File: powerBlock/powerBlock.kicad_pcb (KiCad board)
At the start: 2 copper layers, 3 parts, among them U1 STM32F030C8Tx, U2 74HC164, U3 74HC164

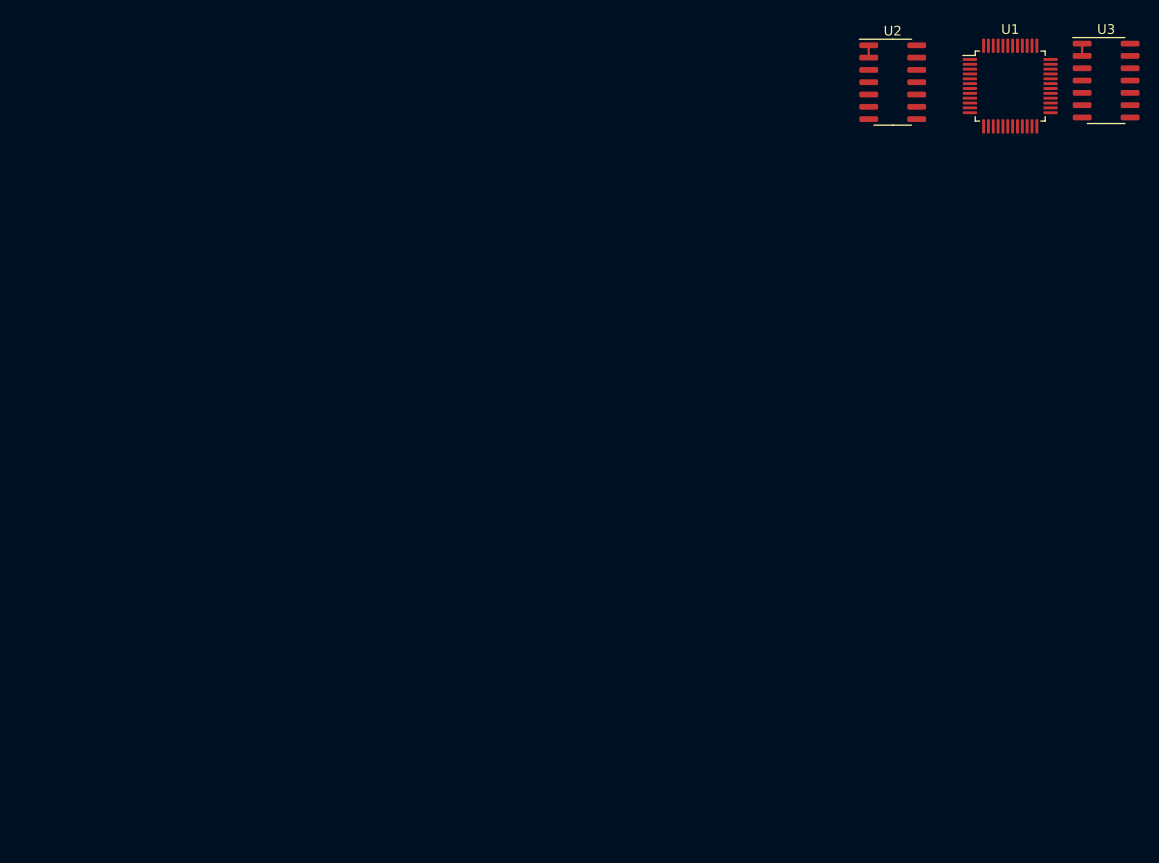
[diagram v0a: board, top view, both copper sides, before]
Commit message: Немного допилил схему. Немного оттрассировал
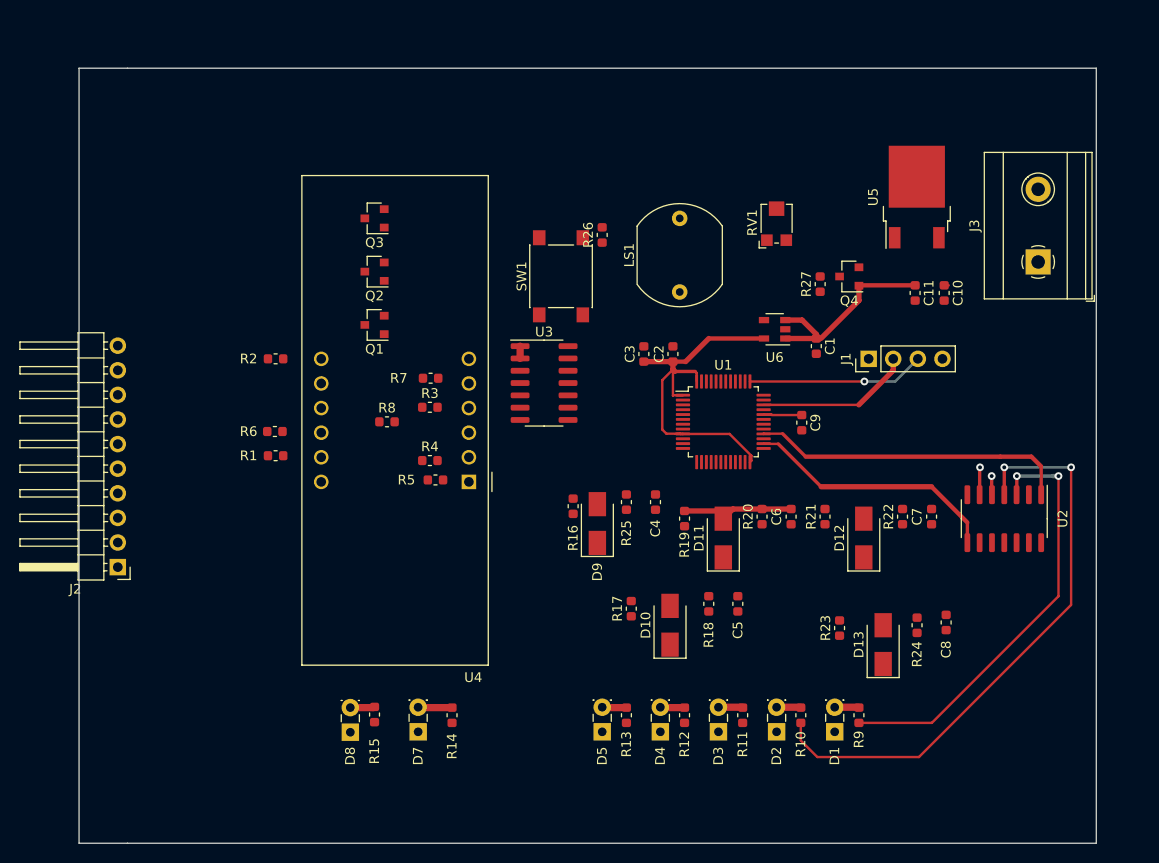
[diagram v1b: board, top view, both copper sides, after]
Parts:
- added C1: 10uF, Capacitor_SMD:C_0603_1608Metric, F.Cu at (111.1, 58.7)
- added C10: 10uF, Capacitor_SMD:C_0603_1608Metric, F.Cu at (124.3, 53.2)
- added C11: 10uF, Capacitor_SMD:C_0603_1608Metric, F.Cu at (121.3, 53.2)
- added C2: 100nF, Capacitor_SMD:C_0603_1608Metric, F.Cu at (96.3, 59.5)
- added C3: 100nF, Capacitor_SMD:C_0603_1608Metric, F.Cu at (93.3, 59.5)
- added C4: 1uF, Capacitor_SMD:C_0603_1608Metric, F.Cu at (94.5, 74.8)
- added C5: 1uF, Capacitor_SMD:C_0603_1608Metric, F.Cu at (103.0, 85.3)
- added C6: 1uF, Capacitor_SMD:C_0603_1608Metric, F.Cu at (108.5, 76.3)
- added C7: 1uF, Capacitor_SMD:C_0603_1608Metric, F.Cu at (123.0, 76.3)
- added C8: 1uF, Capacitor_SMD:C_0603_1608Metric, F.Cu at (124.5, 87.2)
- added C9: 1uF, Capacitor_SMD:C_0603_1608Metric, F.Cu at (109.6, 66.6)
- added D1: LED, LED_THT:LED_Rectangular_W3.9mm_H1.8mm, F.Cu at (113.0, 98.5)
- added D10: DO-214AC, Diode_SMD:D_SMA, F.Cu at (96.0, 87.5)
- added D11: DO-214AC, Diode_SMD:D_SMA, F.Cu at (101.5, 78.5)
- added D12: DO-214AC, Diode_SMD:D_SMA, F.Cu at (116.0, 78.5)
- added D13: DO-214AC, Diode_SMD:D_SMA, F.Cu at (118.0, 89.5)
- added D2: LED, LED_THT:LED_Rectangular_W3.9mm_H1.8mm, F.Cu at (107.0, 98.5)
- added D3: LED, LED_THT:LED_Rectangular_W3.9mm_H1.8mm, F.Cu at (101.0, 98.5)
- added D4: LED, LED_THT:LED_Rectangular_W3.9mm_H1.8mm, F.Cu at (95.0, 98.5)
- added D5: LED, LED_THT:LED_Rectangular_W3.9mm_H1.8mm, F.Cu at (89.0, 98.5)
- added D7: LED, LED_THT:LED_Rectangular_W3.9mm_H1.8mm, F.Cu at (70.0, 98.5)
- added D8: LED, LED_THT:LED_Rectangular_W3.9mm_H1.8mm, F.Cu at (63.0, 98.5)
- added D9: DO-214AC, Diode_SMD:D_SMA, F.Cu at (88.5, 77.0)
- added J1: Conn_01x04, Connector_PinHeader_2.54mm:PinHeader_1x04_P2.54mm_Vertical, F.Cu at (116.5, 60.0)
- added J2: Conn_01x10, Connector_PinHeader_2.54mm:PinHeader_1x10_P2.54mm_Horizontal, F.Cu at (39.0, 81.5)
- added J3: 282844-2, TerminalBlock_MetzConnect:TerminalBlock_MetzConnect_Type175_RT02702HBLC_1x02_P7.50mm_Horizontal, F.Cu at (134.0, 50.0)
- added LS1: Speaker_Crystal, OptoDevice:R_LDR_10x8.5mm_P7.6mm_Vertical, F.Cu at (97.0, 53.1)
- added Q1: BC857BMTF, Package_TO_SOT_SMD:SOT-23, F.Cu at (65.5, 56.5)
- added Q2: BC857BMTF, Package_TO_SOT_SMD:SOT-23, F.Cu at (65.5, 51.0)
- added Q3: BC857BMTF, Package_TO_SOT_SMD:SOT-23, F.Cu at (65.5, 45.5)
- added Q4: BC857BMTF, Package_TO_SOT_SMD:SOT-23, F.Cu at (114.5, 51.5)
- added R1: 18kOhm, Resistor_SMD:R_0603_1608Metric, F.Cu at (55.3, 70.0)
- added R10: 270, Resistor_SMD:R_0603_1608Metric, F.Cu at (109.5, 96.8)
- added R11: 270, Resistor_SMD:R_0603_1608Metric, F.Cu at (103.5, 96.8)
- added R12: 270, Resistor_SMD:R_0603_1608Metric, F.Cu at (97.5, 96.8)
- added R13: 270, Resistor_SMD:R_0603_1608Metric, F.Cu at (91.5, 96.8)
- added R14: 270, Resistor_SMD:R_0603_1608Metric, F.Cu at (73.5, 96.8)
- added R15: 270, Resistor_SMD:R_0603_1608Metric, F.Cu at (65.5, 96.7)
- added R16: 4.3kOhm, Resistor_SMD:R_0603_1608Metric, F.Cu at (86.0, 75.2)
- added R17: 4.3kOhm, Resistor_SMD:R_0603_1608Metric, F.Cu at (92.0, 85.8)
- added R18: 470 Ohm, Resistor_SMD:R_0603_1608Metric, F.Cu at (100.0, 85.3)
- added R19: 4.3kOhm, Resistor_SMD:R_0603_1608Metric, F.Cu at (97.5, 76.5)
- added R2: 18kOhm, Resistor_SMD:R_0603_1608Metric, F.Cu at (55.3, 60.0)
- added R20: 470 Ohm, Resistor_SMD:R_0603_1608Metric, F.Cu at (105.5, 76.3)
- added R21: 4.3kOhm, Resistor_SMD:R_0603_1608Metric, F.Cu at (112.0, 76.3)
- added R22: 470 Ohm, Resistor_SMD:R_0603_1608Metric, F.Cu at (120.0, 76.3)
- added R23: 4.3kOhm, Resistor_SMD:R_0603_1608Metric, F.Cu at (113.5, 87.8)
- added R24: 470 Ohm, Resistor_SMD:R_0603_1608Metric, F.Cu at (121.5, 87.5)
- added R25: 470Ohm, Resistor_SMD:R_0603_1608Metric, F.Cu at (91.5, 74.8)
- added R26: 10kOhm, Resistor_SMD:R_0603_1608Metric, F.Cu at (89.0, 47.2)
- added R27: 330 Ohm, Resistor_SMD:R_0603_1608Metric, F.Cu at (111.5, 52.3)
- added R3: 18kOhm, Resistor_SMD:R_0603_1608Metric, F.Cu at (71.2, 65.0)
- added R4: 18kOhm, Resistor_SMD:R_0603_1608Metric, F.Cu at (71.2, 70.5)
- added R5: 18kOhm, Resistor_SMD:R_0603_1608Metric, F.Cu at (71.8, 72.5)
- added R6: 18kOhm, Resistor_SMD:R_0603_1608Metric, F.Cu at (55.2, 67.5)
- added R7: 18kOhm, Resistor_SMD:R_0603_1608Metric, F.Cu at (71.3, 62.0)
- added R8: 18kOhm, Resistor_SMD:R_0603_1608Metric, F.Cu at (66.8, 66.5)
- added R9: 270, Resistor_SMD:R_0603_1608Metric, F.Cu at (115.5, 96.8)
- added RV1: TC33X-2-502E, Potentiometer_SMD:Potentiometer_Bourns_TC33X_Vertical, F.Cu at (107.0, 46.0)
- added SW1: SW_MEC_5G, Button_Switch_SMD:SW_SPST_PTS645, F.Cu at (84.8, 51.5)
- added U4: BA56-12SRWA, Display_7Segment:CA56-12SEKWA, F.Cu at (75.2, 72.7)
- added U5: LD1086DT50TR, Package_TO_SOT_SMD:TO-252-2, F.Cu at (121.5, 43.3)
- added U6: AP2127K-3.3, Package_TO_SOT_SMD:SOT-23-5, F.Cu at (106.8, 57.0)
- moved U3 65.9 mm to (83.0, 62.5)
- moved U2 46.5 mm to (130.5, 76.5), turned to 270 degrees
- moved U1 45.6 mm to (101.5, 66.5)
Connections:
- U1 pad 1: Net-(U1-Pad1) -> +3V3
- U1 pad 13: Net-(U1-Pad13) -> /ADC3
- U1 pad 14: Net-(U1-Pad14) -> /ADC4
- U1 pad 15: Net-(U1-Pad15) -> /ADC5
- U1 pad 16: Net-(U1-Pad16) -> /ADC6
- U1 pad 17: Net-(U1-Pad17) -> /ADC7
- U1 pad 23: Net-(U1-Pad23) -> GND
- U1 pad 24: Net-(U1-Pad24) -> +3V3
- U1 pad 26: Net-(U1-Pad26) -> /SPI2CLK
- U1 pad 34: Net-(U1-Pad34) -> /SWDIO
- U1 pad 37: Net-(U1-Pad37) -> /SWCLK
- U1 pad 39: Net-(U1-Pad39) -> /SPI1CLK
- U1 pad 40: Net-(U1-Pad40) -> /GPIOB4
- U1 pad 41: Net-(U1-Pad41) -> /SPI1MOSI
- U1 pad 42: Net-(U1-Pad42) -> /GPIOB6
- U1 pad 43: Net-(U1-Pad43) -> /GPIOB7
- U1 pad 45: Net-(U1-Pad45) -> /GPIOB8
- U1 pad 47: Net-(U1-Pad47) -> GND
- U1 pad 48: Net-(U1-Pad48) -> +3V3
- U1 pad 8: Net-(U1-Pad8) -> GND
- U1 pad 9: Net-(U1-Pad9) -> +3V3
- U2 pad 14: Net-(U2-Pad14) -> +5V
- U2 pad 7: Net-(U2-Pad7) -> GND
- U2 pad 8: Net-(U2-Pad8) -> /SPI2CLK
- U2 pad 9: Net-(U2-Pad9) -> +5V
- U3 pad 1: Net-(U3-Pad1) -> /SPI1MOSI
- U3 pad 14: Net-(U3-Pad14) -> +5V
- U3 pad 2: Net-(U3-Pad1) -> /SPI1MOSI
- U3 pad 7: Net-(U3-Pad7) -> GND
- U3 pad 8: Net-(U3-Pad8) -> /SPI1CLK
- U3 pad 9: Net-(U3-Pad9) -> +5V
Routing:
- net Net-(R10-Pad1): track 0.00 -> 60.9 mm, vias 0 -> 2
- net Net-(R9-Pad1): track 0.00 -> 44.7 mm, vias 0 -> 2
- net +3V3: track 0.00 -> 40.6 mm
- net /SPI2MOSI: track 1.27 -> 33.0 mm
- net /SPI2CLK: track 0.00 -> 26.5 mm
- net +5VA: track 0.00 -> 20.8 mm
- net /SWCLK: track 0.00 -> 18.3 mm, vias 0 -> 1
- net /SWDIO: track 0.00 -> 16.0 mm
- net /ADC5: track 0.00 -> 11.7 mm
- net Net-(C9-Pad1): track 0.00 -> 3.99 mm
- net Net-(D7-Pad2): track 0.00 -> 3.52 mm
- net Net-(R12-Pad1): track 0.00 -> 2.84 mm, vias 0 -> 1
- net Net-(D8-Pad2): track 0.00 -> 2.53 mm
- net Net-(D5-Pad2): track 0.00 -> 2.52 mm
- net Net-(D4-Pad2): track 0.00 -> 2.52 mm
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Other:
- board outline added: 105 x 80 mm
